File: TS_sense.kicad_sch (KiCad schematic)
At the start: 33 parts, among them U11 OPA355NA, U13 SFH617A-1X007T, U16 TBA1-0511E

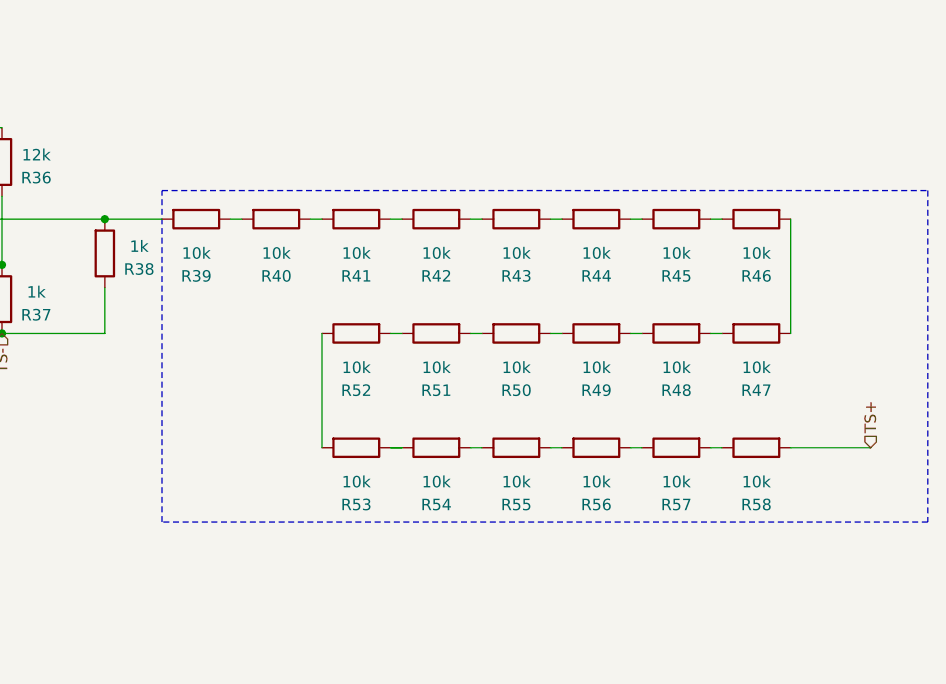
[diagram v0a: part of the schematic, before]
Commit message: Submission Ready. ESF 15.07.24
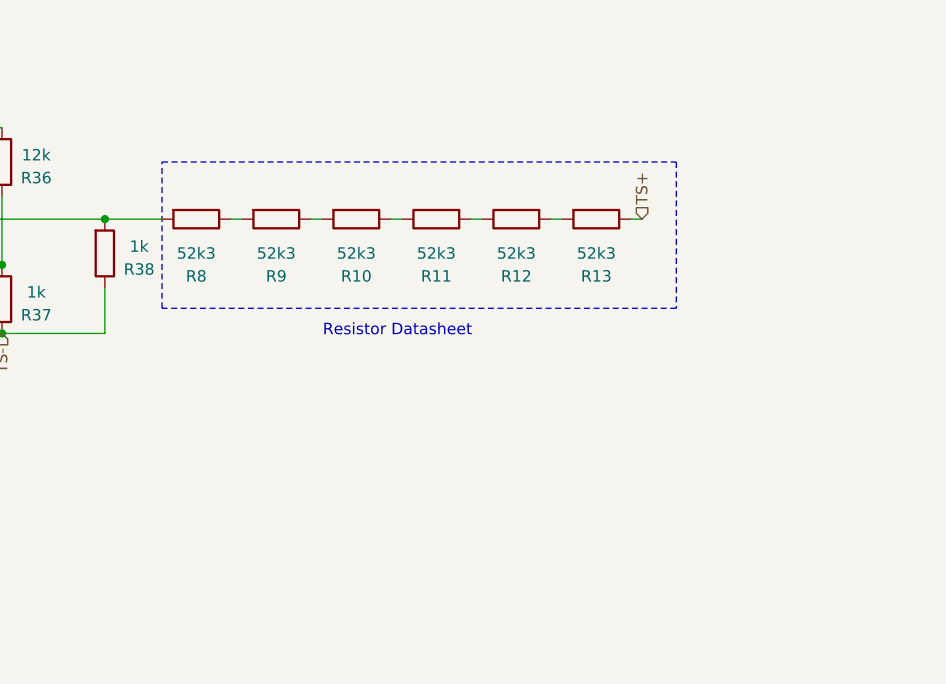
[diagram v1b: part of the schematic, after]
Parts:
- removed R39, R40, R41, R42, R43, R44, R45, R46, R47, R48, R49, R50, R51, R52, R53, R54, R55, R56, R57, R58: 10k, Resistor_SMD:R_0603_1608Metric, symbol Device:R
- added R10, R11, R12, R13, R8, R9: 52k3, Resistor_SMD:R_0805_2012Metric, symbol Device:R
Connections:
- net TS+: now also R13.1
- net at R38.2, U11.3 (+): now also R8.2
- new net: R10.1, R11.1
- new net: R11.2, R12.1
- new net: R12.2, R13.2
- new net: R10.2, R9.1
- new net: R8.1, R9.2
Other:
- note added: "Resistor Datasheet"

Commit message: ⠀⠀⠀⠀⠀⠀⠀⠀⠀⠀⠀⠀⠀⠀⠀⠀⠀⠀⠀⠀⠀⠀⠀⠀⠀⠀⠀⠀⠀⠀⠀⠀⠀⠀⠀⠀⠀⣠⣤⣤⣤⡀⠀⠀⠀⠀⠀⠀⠀⠀⠀⠀⠀⠀⠀⠀⠀⠀⠀⠀⠀⠀⠀⠀⠀ ⠀⠀⠀⠀⠀⠀⠀⠀⠀⠀⠀⠀⠀⠀⠀⠀⠀⠀⠀⠀⠀⠀⠀⠀⠀⠀⠀⠀⠀⠀⠀⠀⠀⠀⣠⣶⣿⠟⠉⠉⠻⣿⡄⠀⠀⠀⠀⠀⠀⠀⠀⠀⠀⠀⠀⠀⠀⠀⠀⠀⠀⠀⠀⠀⠀ ⠀⠀⠀⠀⠀⠀⠀⠀⠀⠀⠀⠀⠀⠀⠀⠀⠀⠀⠀⠀⠀⠀⠀⠀⠀⠀⠀⠀⠀⠀⠀⢀⣤⣾⠿⠉⠀⠀⠀⠀⠀⠹⣿⡄⠀⠀⠀⠀⠀⠀⠀⠀⠀⠀⠀⠀⠀⠀⠀⠀⠀⠀⣀⣴⣾ ⠀⠀⠀⠀⠀⠀⠀⠀⠀⠀⠀⠀⠀⠀⠀⠀⠀⠀⠀⠀⠀⠀⠀⠀⠀⠀⠀⠀⠀⢀⣴⣿⠟⠁⠀⠀⠀⠀⠀⠀⠀⠀⣿⣿⠀⠀⠀⠀⠀⠀⠀⠀⠀⠀⠀⠀⠀⠀⠀⣀⣴⣾⡿⠛⠉ ⠀⠀⠀⠀⠀⠀⠀⠀⠀⠀⠀⠀⠀⠀⠀⠀⠀⠀⠀⠀⠀⠀⠀⠀⠀⠀⠀⢀⣴⣿⠟⠁⠀⠀⠀⠀⠀⠀⠀⠀⠀⠀⢸⣿⡆⠀⠀⠀⠀⠀⠀⠀⠀⠀⠀⠀⢀⣴⣾⡿⠟⠁⠀⠀⠀ ⠀⠀⠀⠀⠀⠀⠀⠀⠀⠀⠀⠀⠀⠀⠀⠀⠀⠀⠀⠀⠀⠀⠀⠀⢀⣀⣴⣿⡿⠃⠀⠀⠀⠀⠀⠀⠀⠀⠀⠀⠀⠀⢸⣿⣷⣶⣶⣦⣤⣤⣄⡀⠀⢀⣠⣾⣿⠿⠋⠀⠀⠀⠀⠀⣠ ⠀⠀⠀⠀⠀⠀⠀⠀⠀⠀⠀⠀⠀⠀⠀⠀⠀⠀⠀⠀⠀⠀⠀⣼⣿⣿⡿⠋⠀⠀⠀⠀⠀⠀⠀⠀⠀⠀⠀⣠⣤⠶⠞⣿⠟⠋⠉⠉⠙⣻⠿⢿⣿⣿⣿⠟⠁⠀⠀⠀⠀⠀⢀⡼⠁ ⠀⠀⠀⠀⠀⠀⠀⠀⠀⠀⠀⠀⠀⠀⠀⠀⠀⠀⠀⠀⠀⠀⢰⣿⠁⠛⠀⠀⠀⠀⠀⠀⠀⠀⠀⠀⠀⠀⣰⠟⠁⢠⡞⠁⠀⠀⠀⢀⡴⠋⠀⢀⡿⠋⠁⠀⠀⠀⠀⠀⠀⠀⡞⠁⠀ ⠀⠀⠀⠀⠀⠀⠀⠀⠀⠀⠀⠀⠀⠀⠀⠀⠀⠀⠀⠀⠀⣠⣼⣿⡄⠀⠀⠀⠀⠀⠀⠀⠀⠀⠀⠀⠀⣼⠃⠀⢠⠏⠀⠀⠀⠀⣰⠏⠀⠀⣠⠟⠀⠀⠀⠀⠀⠀⠀⠀⠀⢸⡥⠤⡀ ⠀⠀⠀⠀⠀⠀⠀⠀⠀⠀⠀⠀⠀⠀⠀⠀⠀⠀⠀⠀⣰⣿⠟⠁⠀⠀⠀⠀⠀⠀⠀⠀⠀⠀⠀⠀⠠⣇⠀⣠⡏⠀⠀⠀⠀⣼⠁⠀⠀⣰⠋⠀⠀⠀⠀⠀⠀⠀⠀⠀⠀⠀⢀⡴⠁ ⠀⠀⠀⠀⠀⠀⠀⠀⠀⠀⠀⠀⠀⠀⠀⠀⣀⣄⣄⣼⣿⠋⠀⠀⠀⠀⠀⠀⠀⠀⠀⠀⠀⠀⠀⠀⠀⢻⡶⠋⠀⠀⠀⠀⢸⣧⠀⠀⣴⠃⠀⠀⠀⠀⠀⠀⠀⠀⠀⠀⠀⠀⠘⢧⠀ ⠀⠀⠀⠀⠀⠀⠀⠀⢀⣀⣀⠀⠀⠀⠀⣾⡿⠿⣿⡿⠁⠀⠀⠀⠀⠀⠀⣠⣶⣶⣶⡀⠀⠀⠀⠀⠀⠀⠀⠀⠀⠀⠀⠀⠀⠙⠛⠛⠁⠀⠀⠀⠀⠀⠀⠀⠀⠀⠀⠀⠀⠀⠀⠈⠳ ⠀⠀⠀⠀⠀⠀⢀⣾⠿⠛⢿⣿⣷⣄⡀⣿⠃⠀⠈⠀⠀⠀⠀⠀⠀⢀⣾⣿⣿⣿⣿⣧⠀⠀⠀⠀⠀⠀⠀⠀⠀⠀⠀⠀⠀⠀⠀⠀⠀⠀⠀⠀⠀⠀⠀⠀⠀⠀⠀⠀⠀⠀⠀⠀⠀ ⠀⠀⠀⣠⣤⣦⣼⣿⠀⠀⠀⣿⣿⣿⣿⣿⣦⣀⠀⠀⠀⠀⠀⠀⠀⣿⣿⣿⣿⣿⣿⡿⠀⠀⠀⢀⣀⣀⣀⣀⡀⠀⠀⠀⠀⠀⠀⠀⠀⠀⠀⣤⣾⣿⣿⣿⣷⣄⠀⠀⠀⠀⠀⠀⠀ ⠀⣠⣾⡿⠋⠉⠉⠁⠀⠀⠀⠀⠉⢯⡙⠻⣿⣿⣷⣤⡀⠀⠀⠀⠀⢿⣿⣿⣿⣿⡿⠃⢀⡤⠖⠋⠉⠉⠉⠉⠉⠉⠒⠦⣄⠀⠀⠀⠀⠀⣾⣿⣿⣿⣿⣿⣿⣿⣧⠀⠀⠀⠀⠀⠀ ⣾⣿⠋⠀⠀⠀⠀⣀⣀⠀⠀⠀⠀⠀⠙⢦⣄⠉⠻⢿⣿⣷⣦⡀⠀⠈⠙⠛⠛⠋⠀⢰⠟⡇⠀⠀⠀⠀⠀⠀⠀⠀⠀⠀⠈⠳⣄⠀⠀⠀⣿⣿⣿⣿⣿⣿⣿⣿⣿⠀⠀⠀⠀⠀⠀ ⣿⡇⠀⠀⠀⣴⠟⣫⣿⣿⣄⠀⠀⠀⠀⡶⢌⡙⠶⣤⡈⠛⠿⣿⣷⣦⣀⠀⠀⠀⠀⡇⠀⢻⣄⠀⠀⣠⢷⠀⠀⠀⠀⠀⡶⠀⠘⡆⠀⠀⠻⣿⣿⣿⣿⣿⣿⣿⡟⠀⠀⠀⠀⠀⠀ ⣿⡇⠀⠀⢸⣟⢸⣿⣿⣿⣿⠀⠀⠀⠀⡇⠀⠈⠛⠦⣝⡳⢤⣈⠛⠻⣿⣷⣦⣀⠀⠀⠀⠀⠈⠙⠋⠁⠀⠛⠦⠤⠤⠚⠁⠀⠀⢳⠀⠀⠀⠈⠛⠿⠿⠿⠟⠋⠀⠀⠀⠀⠀⠀⠀ ⣿⡇⠀⠀⠈⢿⣞⣿⣿⣿⠏⠀⠀⠀⠀⡇⠀⠀⠀⠀⠀⠙⠳⢬⣛⠦⠀⠙⢻⣿⣷⣦⣀⠀⠀⠀⠀⠀⠀⠀⠀⠀⠀⠀⠀⠀⠀⡞⠀⠀⠀⠀⠀⠀⠀⠀⠀⠀⠀⠀⠀⠀⠀⠀⠀ ⣿⡇⠀⠀⠀⠀⠉⠛⠋⠁⠀⠀⠀⠀⠀⡇⠀⠀⠀⠀⠀⠀⠀⠀⠈⠁⠀⠀⠈⣿⠉⢻⣿⣷⣦⣀⠀⠀⠀⠀⠀⠀⠀⠀⠀⢀⡼⠁⠀⠀⠀⠀⠀⠀⠀⠀⠀⠀⠀⠀⠀⠀⠀⠀⠀ ⣿⡇⠀⠀⠀⠀⠀⣠⣄⠀⠀⢰⠶⠒⠒⢧⣄⡀⠀⠀⠀⠀⠀⠀⠀⠀⠀⠀⠀⣿⠀⢸⡇⢸⡟⢿⣷⣦⣴⣶⣶⣶⣶⣤⣔⠋⠀⠀⠀⠀⠀⠀⠀⠀⠀⠀⠀⠀⠀⠀⠀⠀⠀⠀⠀ ⣿⡇⠀⠀⣤⠀⠀⠿⠿⠁⢀⡿⠀⠀⠀⡄⠈⠙⡷⢦⣄⡀⠀⠀⠀⠀⠀⠀⠀⣿⠀⢸⡇⢸⡇⠀⣿⠙⣿⣿⣉⠉⠙⠿⣿⣧⠀⠀⠀⠀⠀⠀⠀⠀⠀⠀⠀⠀⠀⠀⠀⠀⠀⠀⠀ ⣿⡇⠀⠀⠙⠷⢤⣀⣠⠴⠛⠁⠀⠀⠀⠇⠀⠀⡇⢸⡏⢹⡷⢦⣄⡀⠀⠀⠀⣿⡀⢸⡇⢸⡇⠀⡟⠀⢸⠀⢹⡷⢦⣄⣘⣿⡆⠀⠀⠀⠀⠀⠀⠀⠀⠀⠀⠀⠀⠀⠀⠀⠀⠀⠀ ⣿⣿⠢⣤⡀⠀⠀⠀⠀⠀⠀⣠⠾⣿⣿⡷⣤⣀⡇⠸⡇⢸⡇⢸⠉⠙⠳⢦⣄⡻⢿⣾⣧⣸⣧⠀⡇⠀⢸⠀⢸⡇⢤⣈⠙⠻⣿⣆⠀⠀⠀⠀⠀⠀⠀⠀⠀⠀⠀⠀⠀⠀⠀⠀⠀ ⢹⣿⣷⣌⡉⠛⠲⢶⣶⠖⠛⠛⢶⣄⡉⠛⠿⣽⣿⣶⣧⣸⡇⢸⠀⠀⠀⠀⠈⠙⠲⢮⣝⠻⣿⣷⣷⣄⣸⠀⢸⡇⠀⠈⠁⠀⢸⣿⠀⠀⠀⠀⠀⠀⠀⠀⠀⠀⠀⠀⠀⠀⠀⠀⠀ ⠀⠈⠙⠻⢿⣷⣶⣤⣉⡻⢶⣄⣀⠈⠙⠳⢦⣈⡉⠻⢿⣿⣷⣾⣦⡀⠀⠀⠀⠀⠀⠀⠈⠙⠲⢭⣛⠿⣿⣷⣼⡇⠀⠀⠀⠀⠈⣿⡇⠀⠀⠀⠀⠀⠀⣀⠀⠀⠀⠀⠀⠀⠀⠀⣀ ⠀⠀⠀⠀⠀⠈⠙⠻⢿⣿⣷⣶⣽⣻⡦⠀⠀⠈⠙⠷⣦⣌⡙⠻⢿⣟⣷⣤⣀⠀⠀⠀⠀⠀⠀⠀⠈⠙⠳⢯⣻⡇⠀⠀⠀⠀⠀⢸⣿⠀⣀⠀⠀⠀⠀⠈⠳⣄⠀⠀⠀⢀⡏⠙⠛ ⠀⠀⠀⠀⠀⠀⠀⠀⠀⠈⠛⠻⢿⣿⣿⣿⣶⣤⣤⣤⣀⣈⠛⠷⣤⣈⡛⠷⢽⡻⢶⣄⣀⠀⠀⠀⠀⠀⠀⠀⠈⠛⠳⢤⣀⠀⠀⢸⣿⡀⠈⠳⢤⣀⣀⣰⠃⠈⠛⠶⠶⠿⠃⠀⠀ ⠀⠀⠀⠀⠀⠀⠀⠀⠀⠀⠀⠀⠀⢈⣿⡿⠛⠉⠙⠛⠛⠻⢷⣦⣄⣩⣿⠶⠖⠛⠛⠛⠛⠛⠛⠿⢷⣶⣦⣄⠀⠀⠀⠀⠉⢻⣶⣿⣿⠇⠀⠀⠀⠉⠉⠀⠀⠀⠀⠀⠀⠀⠀⠀⠀ ⠀⠀⠀⠀⠀⠀⠀⠀⠀⠀⠀⠀⠀⣼⣿⠁⠀⠀⠀⠀⠀⠀⠀⣿⣿⠋⠀⠀⠀⠀⠀⣠⠖⠂⠀⠀⠀⠈⠙⠿⣿⣦⡄⠀⠀⣸⣿⠟⠋⠀⠀⠀⠀⠀⠀⠀⠀⠀⠀⠀⠀⠀⠀⠀⠀ ⠀⠀⠀⠀⠀⠀⠀⠀⠀⠀⠀⠀⢰⣿⡟⠀⠀⠀⠀⠀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
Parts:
- C39, C40, C41, C42: footprint (none) -> Capacitor_SMD:C_0603_1608Metric
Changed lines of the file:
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@@
 			)
 		)
-		(property "Footprint" ""
+		(property "Footprint" "Capacitor_SMD:C_0603_1608Metric"
 			(at 115.2652 58.42 0)
 			(effects
@@
 			)
 		)
-		(property "Footprint" ""
+		(property "Footprint" "Capacitor_SMD:C_0603_1608Metric"
 			(at 62.5348 58.42 0)
 			(effects
@@
 			)
 		)
-		(property "Footprint" ""
+		(property "Footprint" "Capacitor_SMD:C_0603_1608Metric"
 			(at 49.8348 58.42 0)
 			(effects
@@
 			)
 		)
-		(property "Footprint" ""
+		(property "Footprint" "Capacitor_SMD:C_0603_1608Metric"
 			(at 102.5652 58.42 0)
 			(effects

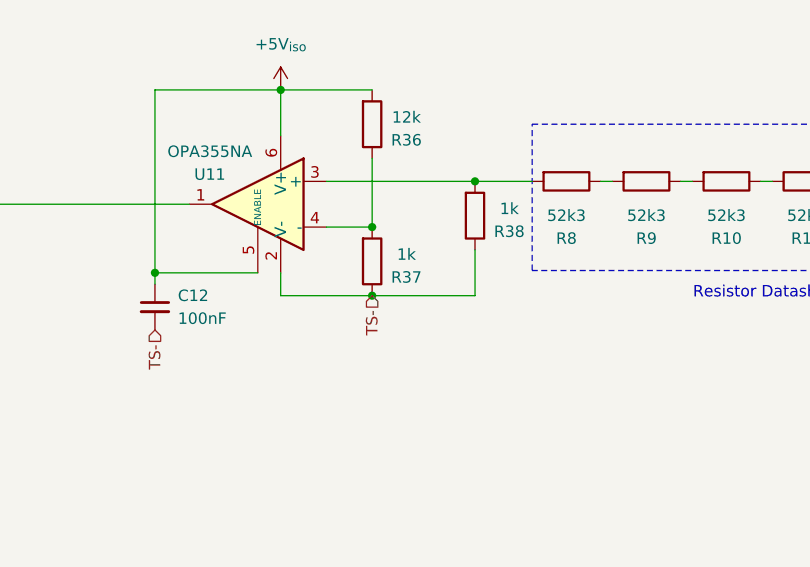
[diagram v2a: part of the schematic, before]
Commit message: TSAL Rev 0.2
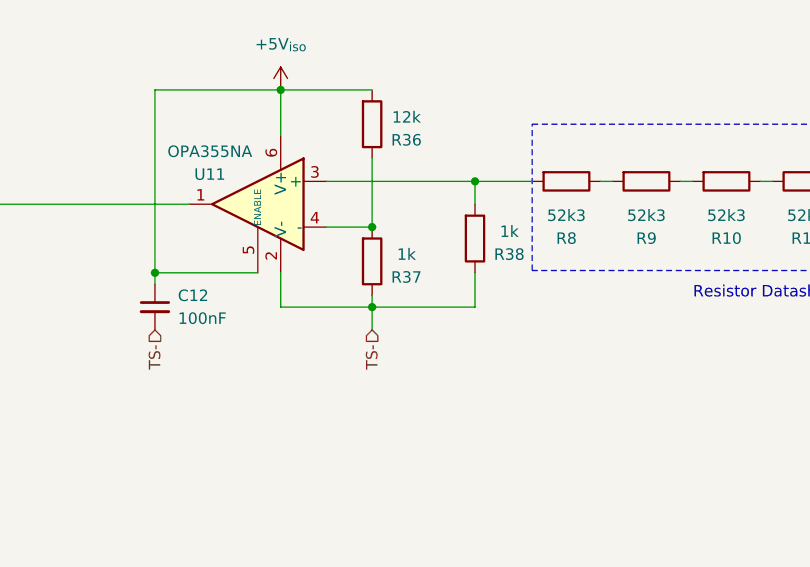
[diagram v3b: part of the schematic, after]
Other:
- moved on the sheet: R38
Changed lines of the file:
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@@
 		(title "TSAL")
 		(date "2024-07-11")
-		(rev "V0.1")
+		(rev "V0.2")
 		(company "Team RPM - UAS Münster")
 		(comment 1 "Luca Sapion")
@@
 	)
 	(junction
-		(at 138.43 96.52)
-		(diameter 0)
-		(color 0 0 0 0)
-	)
-	(junction
 		(at 71.12 91.44)
 		(diameter 0)
@@
 	)
 	(junction
+		(at 138.43 97.79)
+		(diameter 0)
+		(color 0 0 0 0)
+	)
+	(junction
 		(at 101.6 50.8)
 		(diameter 0)
@@
 	(wire
 		(pts
+			(xy 138.43 97.79) (xy 138.43 96.52)
+		)
+		(stroke
+			(width 0)
+			(type default)
+		)
+	)
+	(wire
+		(pts
 			(xy 92.71 50.8) (xy 101.6 50.8)
 		)
@@
 	(wire
 		(pts
+			(xy 138.43 100.33) (xy 138.43 97.79)
+		)
+		(stroke
+			(width 0)
+			(type default)
+		)
+	)
+	(wire
+		(pts
+			(xy 149.86 86.36) (xy 149.86 83.82)
+		)
+		(stroke
+			(width 0)
+			(type default)
+		)
+	)
+	(wire
+		(pts
 			(xy 125.73 93.98) (xy 114.3 93.98)
 		)
@@
 	(wire
 		(pts
-			(xy 128.27 93.98) (xy 128.27 96.52)
+			(xy 128.27 93.98) (xy 128.27 97.79)
 		)
 		(stroke
@@
 	(wire
 		(pts
-			(xy 128.27 96.52) (xy 138.43 96.52)
+			(xy 128.27 97.79) (xy 138.43 97.79)
 		)
 		(stroke
@@
 	(wire
 		(pts
-			(xy 138.43 96.52) (xy 149.86 96.52)
+			(xy 138.43 97.79) (xy 149.86 97.79)
 		)
 		(stroke
@@
 	(wire
 		(pts
-			(xy 149.86 96.52) (xy 149.86 91.44)
+			(xy 149.86 97.79) (xy 149.86 93.98)
 		)
 		(stroke
@@
 	(hierarchical_label "TS-"
 		(shape input)
-		(at 138.43 96.52 270)
+		(at 138.43 100.33 270)
 		(fields_autoplaced yes)
 		(effects
@@
 	(symbol
 		(lib_id "Device:R")
-		(at 149.86 87.63 0)
+		(at 149.86 90.17 0)
 		(mirror x)
 		(unit 1)
@@
 		(dnp no)
 		(property "Reference" "R38"
+			(at 153.67 91.948 0)
+			(effects
+				(font
+					(size 1.27 1.27)
+				)
+			)
+		)
+		(property "Value" "1k"
 			(at 153.67 89.408 0)
 			(effects
@@
 			)
 		)
-		(property "Value" "1k"
-			(at 153.67 86.868 0)
-			(effects
-				(font
-					(size 1.27 1.27)
-				)
-			)
-		)
 		(property "Footprint" "Resistor_SMD:R_0603_1608Metric"
-			(at 148.082 87.63 90)
+			(at 148.082 90.17 90)
 			(effects
 				(font
@@
 		)
 		(property "Datasheet" "~"
-			(at 149.86 87.63 0)
+			(at 149.86 90.17 0)
 			(effects
 				(font
@@
 		)
 		(property "Description" "Resistor"
-			(at 149.86 87.63 0)
-			(effects
-				(font
+			(at 149.86 90.17 0)
+			(effects
+				(font
